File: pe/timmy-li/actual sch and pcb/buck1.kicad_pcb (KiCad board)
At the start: 2 copper layers, 6 parts, among them U1 TPS62143

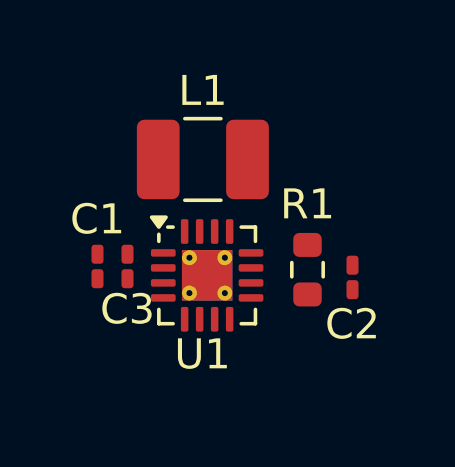
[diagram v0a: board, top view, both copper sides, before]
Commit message: fixed pcb
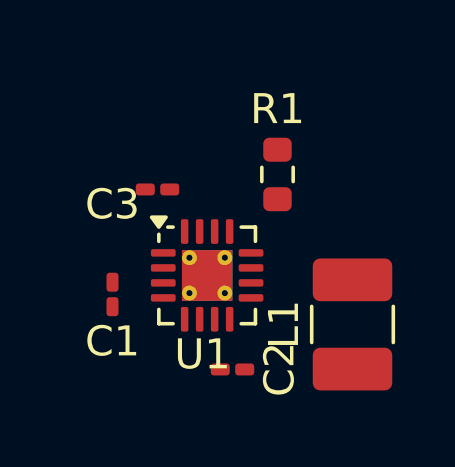
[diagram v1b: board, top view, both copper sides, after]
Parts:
- moved L1 7.42 mm to (119.5, 104.5), turned to 90 degrees
- moved C2 5.04 mm to (115.5, 106.0), turned to 0 degrees
- moved R1 3.33 mm to (117.0, 99.5)
- moved C3 2.76 mm to (113.0, 100.0), turned to 180 degrees
- moved C1 1.06 mm to (111.5, 103.5), turned to -90 degrees
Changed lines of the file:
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@@
 	(footprint "Resistor_SMD:R_0603_1608Metric"
 		(layer "F.Cu")
-		(at 118 102.675 -90)
+		(at 117 99.5 -90)
 		(descr "Resistor SMD 0603 (1608 Metric), square (rectangular) end terminal, IPC-7351 nominal, (Body size source: IPC-SM-782 page 72, https://www.pcb-3d.com/wordpress/wp-content/uploads/ipc-sm-782a_amendment_1_and_2.pdf)")
 		(tags "resistor")
@@
 	(footprint "Capacitor_SMD:C_0201_0603Metric_Pad0.64x0.40mm_HandSolder"
 		(layer "F.Cu")
-		(at 112 102.5675 90)
+		(at 113 100 180)
 		(descr "Capacitor SMD 0201 (0603 Metric), square (rectangular) end terminal, IPC-7351 nominal with elongated pad for handsoldering. (Body size source: https://www.vishay.com/docs/20052/crcw0201e3.pdf)")
 		(tags "capacitor handsolder")
 		(property "Reference" "C3"
-			(at -1.4325 0 180)
+			(at 1.5 -0.5 180)
 			(layer "F.SilkS")
 			(effects
@@
 		)
 		(property "Value" "3.3nF"
-			(at 0 1.05 90)
+			(at 0 1.05 0)
 			(layer "F.Fab")
 			(effects
@@
 		)
 		(property "Datasheet" ""
-			(at 0 0 90)
+			(at 0 0 0)
 			(layer "F.Fab")
 			(hide yes)
@@
 		)
 		(property "Description" "Unpolarized capacitor, small symbol"
-			(at 0 0 90)
+			(at 0 0 0)
 			(layer "F.Fab")
 			(hide yes)
@@
 		)
 		(property "KiLib_Generator" "SMD_2terminal_chip_molded"
-			(at 0 0 90)
+			(at 0 0 0)
 			(layer "F.SilkS")
 			(hide yes)
@@
 		)
 		(fp_text user "${REFERENCE}"
-			(at 0 -0.68 90)
+			(at 0 -0.68 0)
 			(layer "F.Fab")
 			(effects
@@
 		)
 		(pad "" smd roundrect
-			(at -0.4325 0 90)
+			(at -0.4325 0 180)
 			(size 0.458 0.36)
 			(layers "F.Paste")
@@
 		)
 		(pad "" smd roundrect
-			(at 0.4325 0 90)
+			(at 0.4325 0 180)
 			(size 0.458 0.36)
 			(layers "F.Paste")
@@
 		)
 		(pad "1" smd roundrect
-			(at -0.4075 0 90)
+			(at -0.4075 0 180)
 			(size 0.635 0.4)
 			(layers "F.Cu" "F.Mask")
@@
 		)
 		(pad "2" smd roundrect
-			(at 0.4075 0 90)
+			(at 0.4075 0 180)
 			(size 0.635 0.4)
 			(layers "F.Cu" "F.Mask")
@@
 		)
 		(property "Value" "TPS62143"
-			(at 0 2.83 0)
+			(at 0 3.135 0)
 			(layer "F.Fab")
 			(effects
@@
 	(footprint "Capacitor_SMD:C_0201_0603Metric_Pad0.64x0.40mm_HandSolder"
 		(layer "F.Cu")
-		(at 111 102.5675 90)
+		(at 111.5 103.5 -90)
 		(descr "Capacitor SMD 0201 (0603 Metric), square (rectangular) end terminal, IPC-7351 nominal with elongated pad for handsoldering. (Body size source: https://www.vishay.com/docs/20052/crcw0201e3.pdf)")
 		(tags "capacitor handsolder")
 		(property "Reference" "C1"
-			(at 1.5675 0 180)
+			(at 1.5675 0 0)
 			(layer "F.SilkS")
 			(effects
@@
 		)
 		(property "Digikey Part Number" ""
-			(at 0 0 90)
+			(at 0 0 270)
 			(unlocked yes)
 			(layer "F.Fab")
@@
 		)
 		(property "Digikey URL" ""
-			(at 0 0 90)
+			(at 0 0 270)
 			(unlocked yes)
 			(layer "F.Fab")
@@
 		)
 		(property "Manufacturer" ""
-			(at 0 0 90)
+			(at 0 0 270)
 			(unlocked yes)
 			(layer "F.Fab")
@@
 		)
 		(property "Manufacturer Part Number" ""
-			(at 0 0 90)
+			(at 0 0 270)
 			(unlocked yes)
 			(layer "F.Fab")
@@
 		)
 		(pad "" smd roundrect
-			(at -0.4325 0 90)
+			(at -0.4325 0 270)
 			(size 0.458 0.36)
 			(layers "F.Paste")
@@
 		)
 		(pad "" smd roundrect
-			(at 0.4325 0 90)
+			(at 0.4325 0 270)
 			(size 0.458 0.36)
 			(layers "F.Paste")
@@
 		)
 		(pad "1" smd roundrect
-			(at -0.4075 0 90)
+			(at -0.4075 0 270)
 			(size 0.635 0.4)
 			(layers "F.Cu" "F.Mask")
@@
 		)
 		(pad "2" smd roundrect
-			(at 0.4075 0 90)
+			(at 0.4075 0 270)
 			(size 0.635 0.4)
 			(layers "F.Cu" "F.Mask")
@@
 	(footprint "Inductor_SMD:L_1210_3225Metric_Pad1.42x2.65mm_HandSolder"
 		(layer "F.Cu")
-		(at 114.5125 99)
+		(at 119.5 104.5 90)
 		(descr "Inductor SMD 1210 (3225 Metric), square (rectangular) end terminal, IPC-7351 nominal with elongated pad for handsoldering. (Body size source: http://www.tortai-tech.com/upload/download/2011102023233369053.pdf)")
 		(tags "inductor handsolder")
 		(property "Reference" "L1"
-			(at 0 -2.28 0)
+			(at 0 -2.28 90)
 			(layer "F.SilkS")
 			(effects
@@
 		)
 		(property "Value" "2.2uH"
-			(at 0 2.28 0)
+			(at 0 2.28 90)
 			(layer "F.Fab")
 			(effects
@@
 		)
 		(property "Datasheet" ""
-			(at 0 0 0)
+			(at 0 0 90)
 			(layer "F.Fab")
 			(hide yes)
@@
 		)
 		(property "Description" "Inductor, small symbol"
-			(at 0 0 0)
+			(at 0 0 90)
 			(layer "F.Fab")
 			(hide yes)
@@
 		)
 		(property "KiLib_Generator" "SMD_2terminal_chip_molded"
-			(at 0 0 0)
+			(at 0 0 90)
 			(layer "F.SilkS")
 			(hide yes)
@@
 		)
 		(property "Digikey Part Number" ""
-			(at 0 0 0)
+			(at 0 0 90)
 			(unlocked yes)
 			(layer "F.Fab")
@@
 		)
 		(property "Digikey URL" ""
-			(at 0 0 0)
+			(at 0 0 90)
 			(unlocked yes)
 			(layer "F.Fab")
@@
 		)
 		(property "Manufacturer" ""
-			(at 0 0 0)
+			(at 0 0 90)
 			(unlocked yes)
 			(layer "F.Fab")
@@
 		)
 		(property "Manufacturer Part Number" ""
-			(at 0 0 0)
+			(at 0 0 90)
 			(unlocked yes)
 			(layer "F.Fab")
@@
 		)
 		(fp_text user "${REFERENCE}"
-			(at 0 0 0)
+			(at 0 0 90)
 			(layer "F.Fab")
 			(effects
@@
 		)
 		(pad "1" smd roundrect
-			(at -1.4875 0)
+			(at -1.4875 0 90)
 			(size 1.425 2.65)
 			(layers "F.Cu" "F.Mask" "F.Paste")
@@
 		)
 		(pad "2" smd roundrect
-			(at 1.4875 0)
+			(at 1.4875 0 90)
 			(size 1.425 2.65)
 			(layers "F.Cu" "F.Mask" "F.Paste")
@@
 	(footprint "Capacitor_SMD:C_0201_0603Metric_Pad0.64x0.40mm_HandSolder"
 		(layer "F.Cu")
-		(at 119.5 102.9325 -90)
+		(at 115.5 106)
 		(descr "Capacitor SMD 0201 (0603 Metric), square (rectangular) end terminal, IPC-7351 nominal with elongated pad for handsoldering. (Body size source: https://www.vishay.com/docs/20052/crcw0201e3.pdf)")
 		(tags "capacitor handsolder")
 		(property "Reference" "C2"
-			(at 1.5675 0 180)
+			(at 1.5675 0 90)
 			(layer "F.SilkS")
 			(effects
@@
 		)
 		(property "Value" "22uF"
-			(at 0 1.05 90)
+			(at 0 1.05 0)
 			(layer "F.Fab")
 			(effects
@@
 		)
 		(property "Datasheet" ""
-			(at 0 0 90)
+			(at 0 0 0)
 			(layer "F.Fab")
 			(hide yes)
@@
 		)
 		(property "Description" "Unpolarized capacitor, small symbol"
-			(at 0 0 90)
+			(at 0 0 0)
 			(layer "F.Fab")
 			(hide yes)
@@
 		)
 		(property "KiLib_Generator" "SMD_2terminal_chip_molded"
-			(at 0 0 90)
+			(at 0 0 0)
 			(layer "F.SilkS")
 			(hide yes)
@@
 		)
 		(property "Digikey Part Number" ""
-			(at 0 0 270)
+			(at 0 0 0)
 			(unlocked yes)
 			(layer "F.Fab")
@@
 		)
 		(property "Digikey URL" ""
-			(at 0 0 270)
+			(at 0 0 0)
 			(unlocked yes)
 			(layer "F.Fab")
@@
 		)
 		(property "Manufacturer" ""
-			(at 0 0 270)
+			(at 0 0 0)
 			(unlocked yes)
 			(layer "F.Fab")
@@
 		)
 		(property "Manufacturer Part Number" ""
-			(at 0 0 270)
+			(at 0 0 0)
 			(unlocked yes)
 			(layer "F.Fab")
@@
 		)
 		(fp_text user "${REFERENCE}"
-			(at 0 -0.68 90)
+			(at 0 -0.68 0)
 			(layer "F.Fab")
 			(effects
@@
 		)
 		(pad "" smd roundrect
-			(at -0.4325 0 270)
+			(at -0.4325 0)
 			(size 0.458 0.36)
 			(layers "F.Paste")
@@
 		)
 		(pad "" smd roundrect
-			(at 0.4325 0 270)
+			(at 0.4325 0)
 			(size 0.458 0.36)
 			(layers "F.Paste")
@@
 		)
 		(pad "1" smd roundrect
-			(at -0.4075 0 270)
+			(at -0.4075 0)
 			(size 0.635 0.4)
 			(layers "F.Cu" "F.Mask")
@@
 		)
 		(pad "2" smd roundrect
-			(at 0.4075 0 270)
+			(at 0.4075 0)
 			(size 0.635 0.4)
 			(layers "F.Cu" "F.Mask")
